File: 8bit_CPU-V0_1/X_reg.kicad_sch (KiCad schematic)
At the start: 5 parts, among them U26 74LS04, U60 74LS04, U61 74LS574

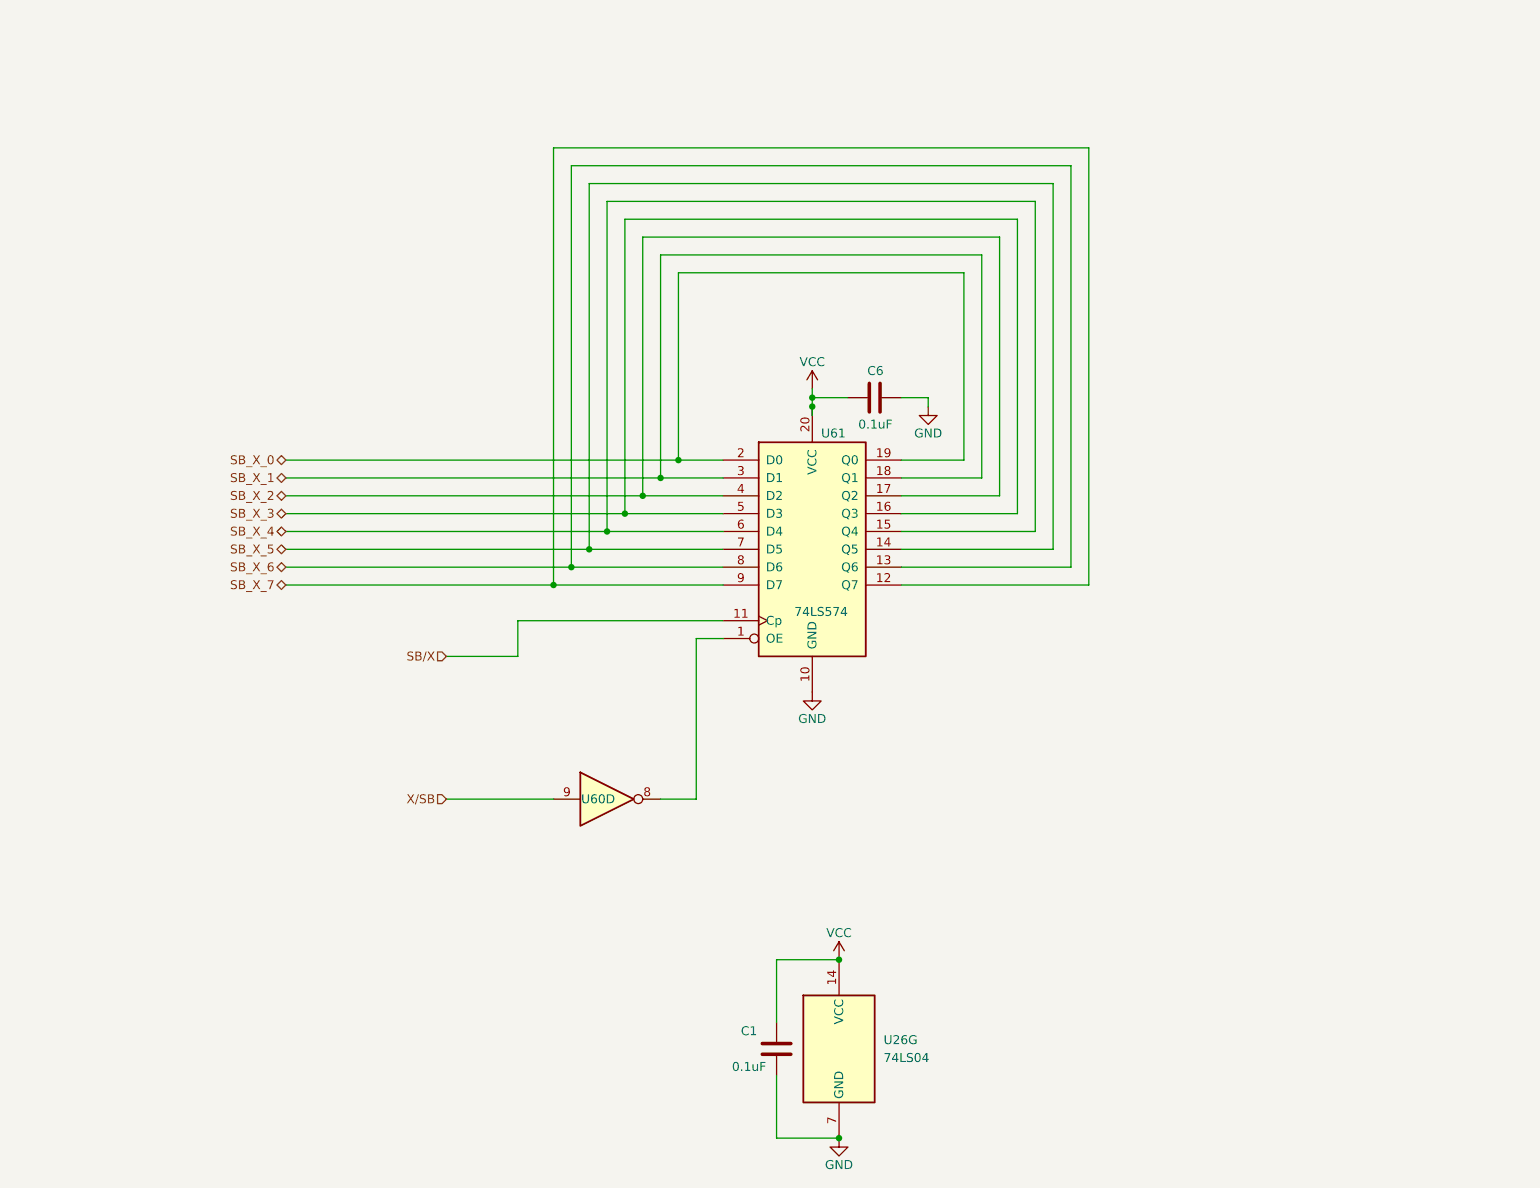
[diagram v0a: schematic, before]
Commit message: Update
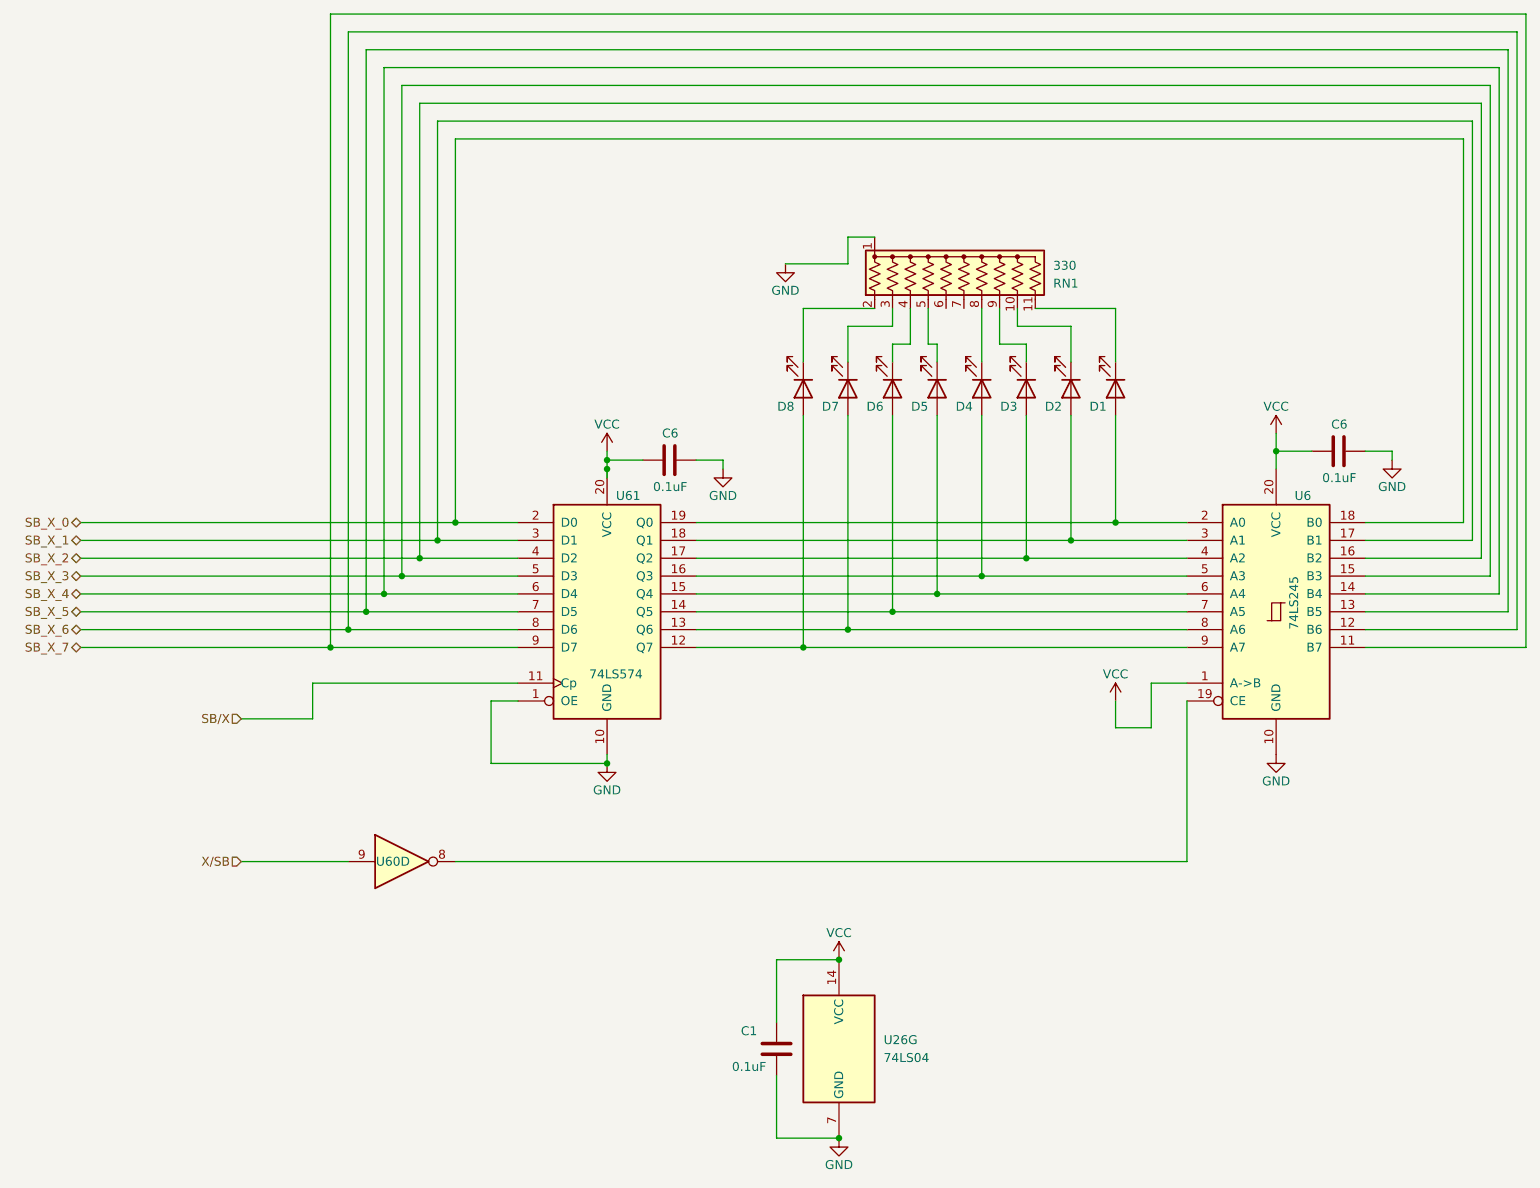
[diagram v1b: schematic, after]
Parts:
- added C6: 0.1uF, symbol Device:C
- added D1, D2, D3, D4, D5, D6, D7, D8: LED, symbol Device:LED
- added RN1: 330, Resistor_THT:R_Array_SIP11, symbol Device:R_Network10_US
- added U6: 74LS245, symbol 74xx:74LS245
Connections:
- net GND: now also U61.1 (OE), C6.2, RN1.1 (common), U6.10 (GND)
- net SB_X_0: now also U6.18 (B0); no longer U61.19 (Q0)
- net SB_X_1: now also U6.17 (B1); no longer U61.18 (Q1)
- net SB_X_2: now also U6.16 (B2); no longer U61.17 (Q2)
- net SB_X_3: now also U6.15 (B3); no longer U61.16 (Q3)
- net SB_X_4: now also U6.14 (B4); no longer U61.15 (Q4)
- net SB_X_5: now also U6.13 (B5); no longer U61.14 (Q5)
- net SB_X_6: now also U6.12 (B6); no longer U61.13 (Q6)
- net SB_X_7: now also U6.11 (B7); no longer U61.12 (Q7)
- net VCC: now also C6.1, U6.1 (A->B), U6.20 (VCC)
- net at U60.8: now also U6.19 (CE); no longer U61.1 (OE)
- new net: D8.1 (K), RN1.2 (R1)
- new net: D8.2 (A), U6.9 (A7), U61.12 (Q7)
- new net: D4.1 (K), RN1.8 (R7)
- new net: D4.2 (A), U6.5 (A3), U61.16 (Q3)
- new net: D2.1 (K), RN1.10 (R9)
- new net: D2.2 (A), U6.3 (A1), U61.18 (Q1)
- new net: D7.1 (K), RN1.3 (R2)
- new net: D7.2 (A), U6.8 (A6), U61.13 (Q6)
- new net: D1.2 (A), U6.2 (A0), U61.19 (Q0)
- new net: D3.2 (A), U6.4 (A2), U61.17 (Q2)
- new net: D5.2 (A), U6.6 (A4), U61.15 (Q4)
- new net: D6.2 (A), U6.7 (A5), U61.14 (Q5)
- new net: D6.1 (K), RN1.4 (R3)
- new net: D3.1 (K), RN1.9 (R8)
- new net: D1.1 (K), RN1.11 (R10)
- new net: D5.1 (K), RN1.5 (R4)
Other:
- moved on the sheet: C6, U60D, U61
